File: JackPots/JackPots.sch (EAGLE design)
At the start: 20 parts, among them J101 F10, J102 F10, P1J0 JACK-3_5MM-MONO-SW-WQP_PJ302-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, P1JI JACK-3_5MM-MONO-SW-WQP_PJ302-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, P2J0 JACK-3_5MM-MONO-SW-WQP_PJ302-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, P2JI JACK-3_5MM-MONO-SW-WQP_PJ302-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, P3JI JACK-3_5MM-MONO-SW-WQP_PJ302-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, P3JO JACK-3_5MM-MONO-SW-WQP_PJ302-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, P4JI JACK-3_5MM-MONO-SW-WQP_PJ302-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, P4JO JACK-3_5MM-MONO-SW-WQP_PJ302-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

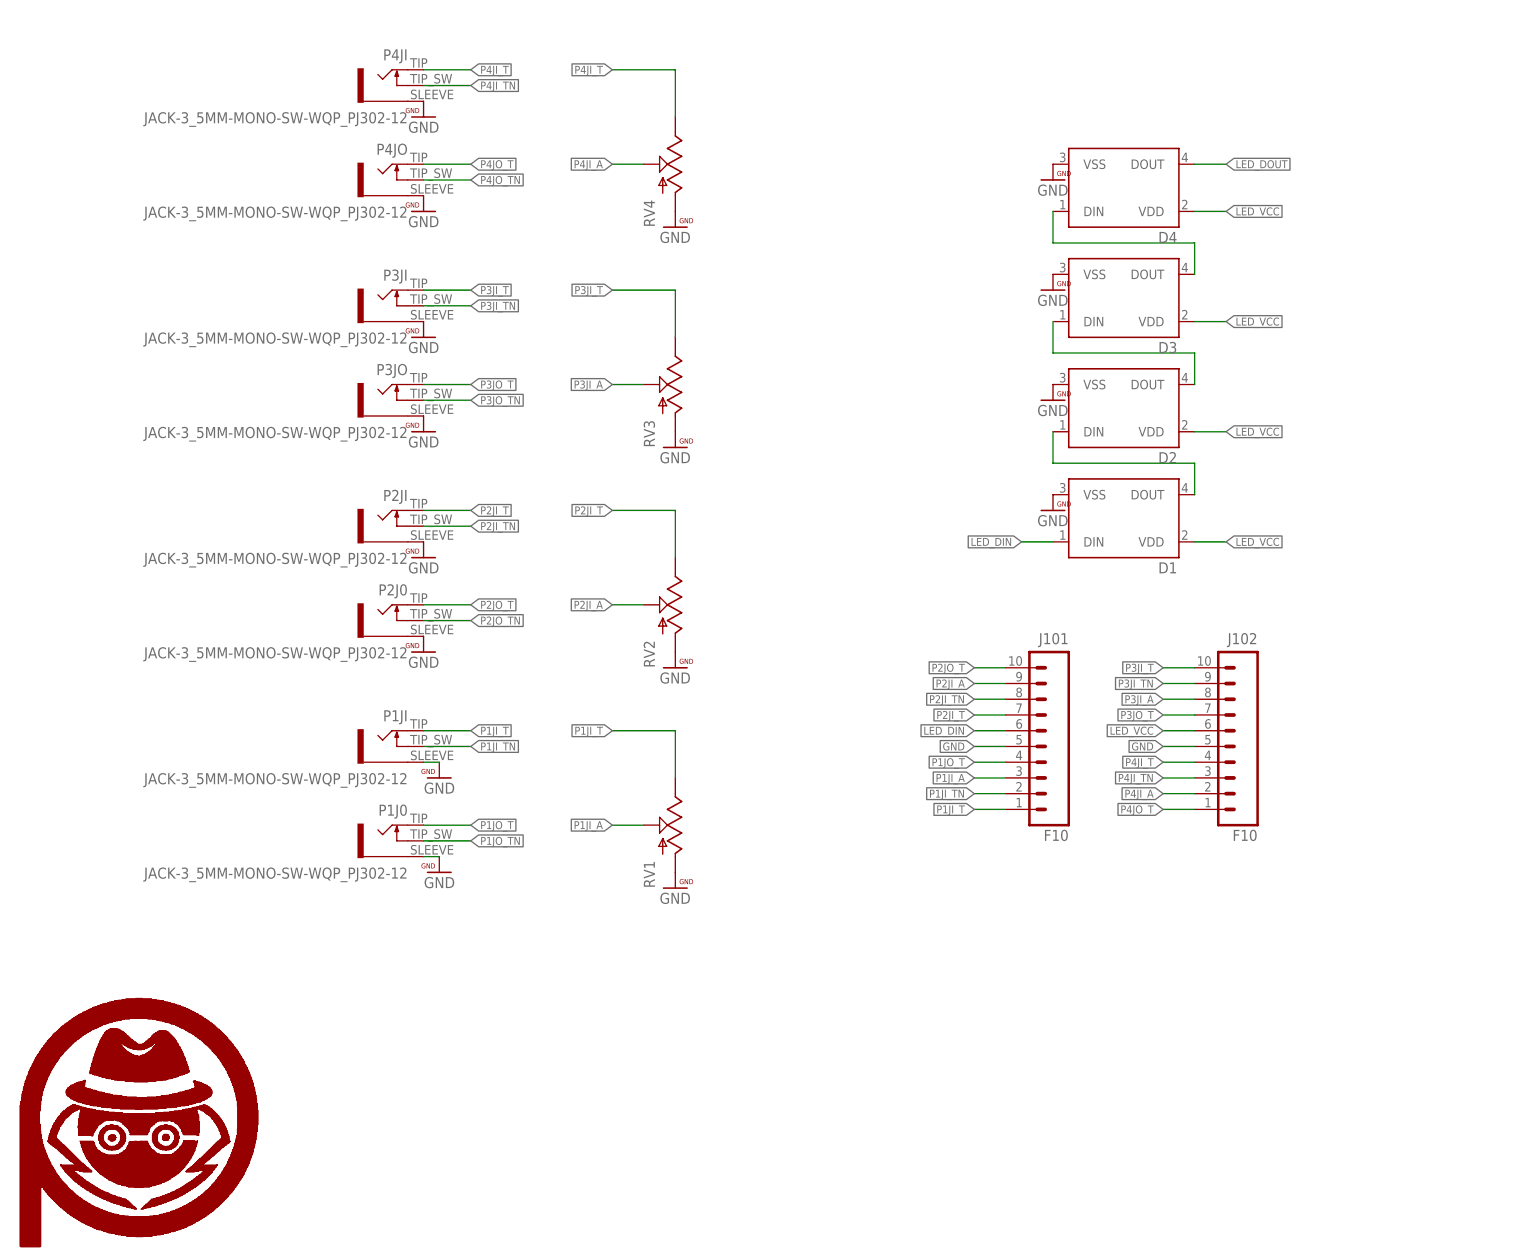
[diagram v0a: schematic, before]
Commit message: 4/10 update
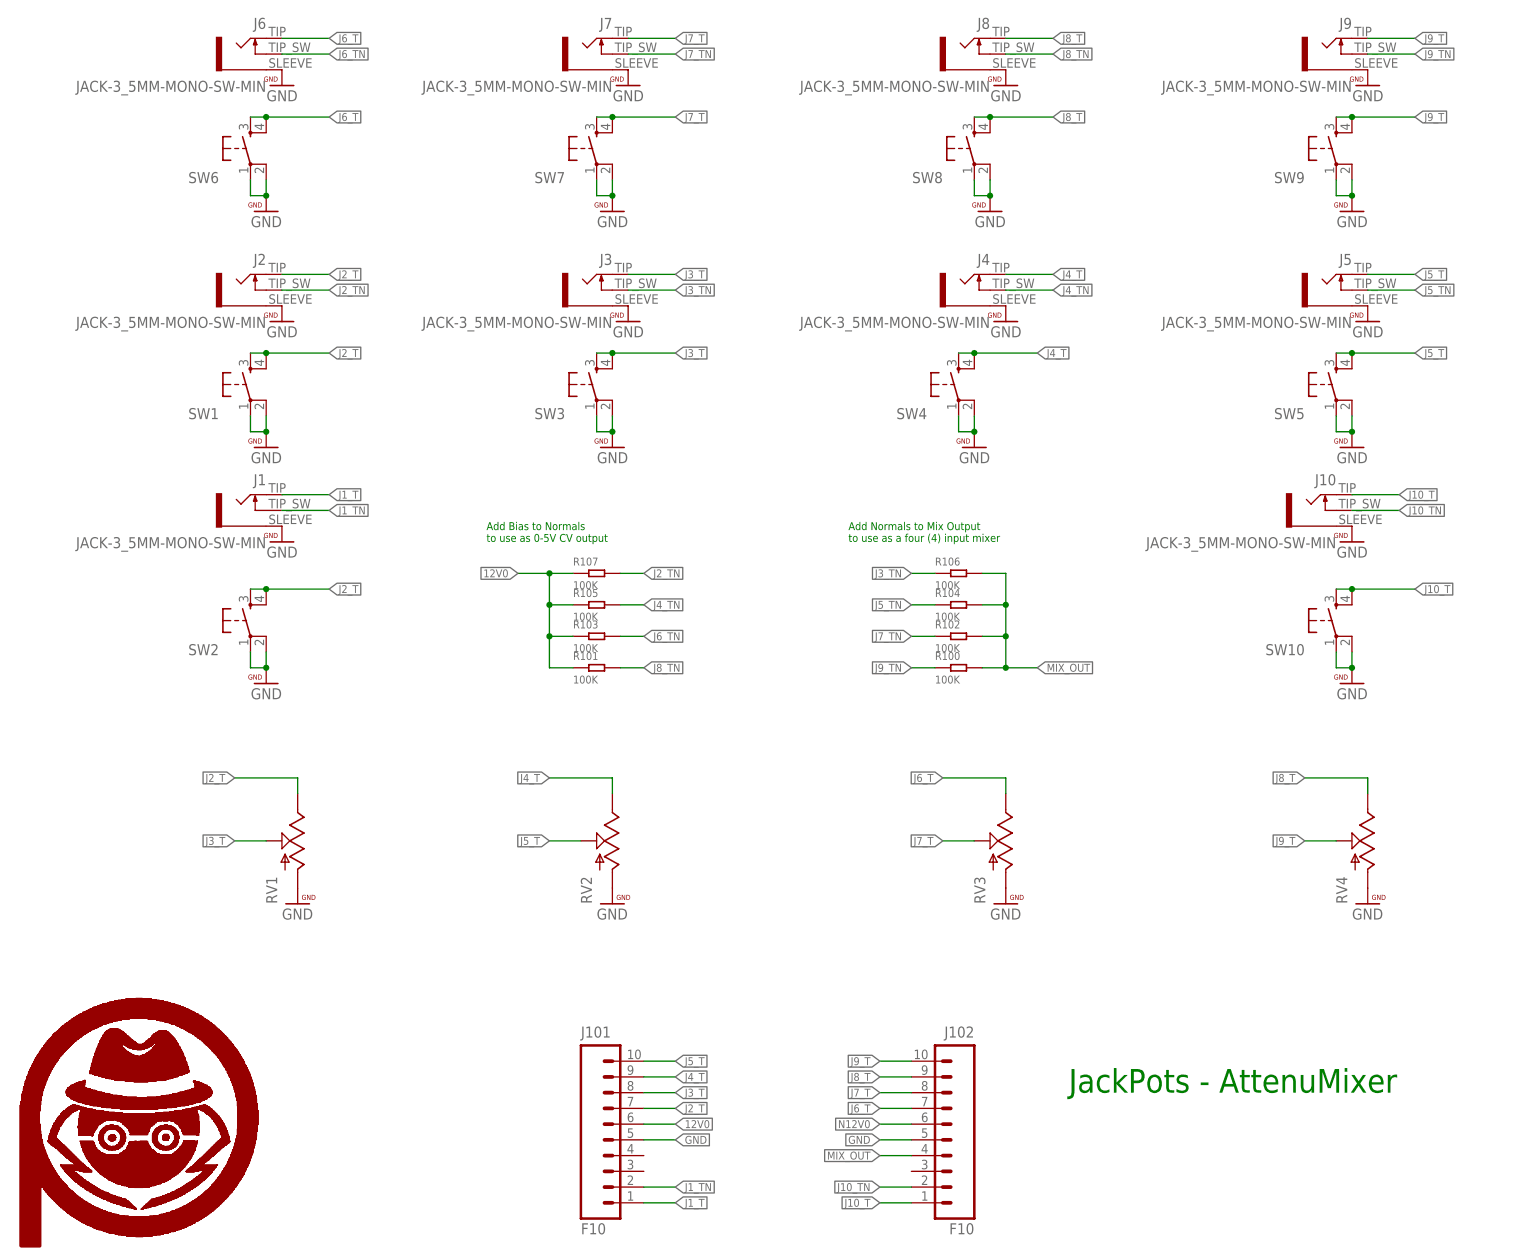
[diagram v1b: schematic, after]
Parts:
- removed D1, D2, D3, D4: (no value), halcyonmod_Optoelectronics:WS2812B-PTH
- removed P1J0, P1JI, P2J0, P2JI, P3JI, P3JO, P4JI, P4JO: JACK-3_5MM-MONO-SW-WQP_PJ302-12, oXo_Connectors:JACK-3_5MM-MONO-SW-WQP_PJ302-12
- removed U$16, U$18: PA_LOGO_SYMMED, PatternAgents-Logos:PA_LOGO_SYMMED
- added $$U$1: PA_LOGO_SYMSMALL, PatternAgents-Logos:PA_LOGO_SYMSMALL
- added $$U$100, $$U$101: PA_LOGO_SYMMED, PatternAgents-Logos:PA_LOGO_SYMMED
- added J1, J10, J2, J3, J4, J5, J6, J7, J8, J9: JACK-3_5MM-MONO-SW-MIN, halcyonmod_Connectors:JACK-3_5MM-MONO-SW-MIN
- added R100, R101, R102, R103, R104, R105, R106, R107: 100K, Seeed-Resistor-2016:SMD-RES-100K-1%-1/10W(0603)
- added SW1, SW10, SW2, SW3, SW4, SW5, SW6, SW7, SW8, SW9: (no value), SparkFun:TAC_SWITCHPTH
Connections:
- removed net LED_DIN: D1.DIN, J101.6
- removed net LED_DOUT: D4.DOUT
- removed net LED_VCC: D1.VDD, D2.VDD, D3.VDD, D4.VDD, J102.6
- removed net N$1: D1.DOUT, D2.DIN
- removed net N$2: D2.DOUT, D3.DIN
- removed net N$3: D3.DOUT, D4.DIN
- removed net P1JI_A: J101.3, RV1.2
- removed net P1JI_T: J101.1, P1JI.TIP, RV1.3
- removed net P1JI_TN: J101.2, P1JI.TIP_SW
- removed net P1JO_T: J101.4, P1J0.TIP
- removed net P1JO_TN: P1J0.TIP_SW
- removed net P2JI_A: J101.9, RV2.2
- removed net P2JI_T: J101.7, P2JI.TIP, RV2.3
- removed net P2JI_TN: J101.8, P2JI.TIP_SW
- removed net P2JO_T: J101.10, P2J0.TIP
- removed net P2JO_TN: P2J0.TIP_SW
- removed net P3JI_A: J102.8, RV3.2
- removed net P3JI_T: J102.10, P3JI.TIP, RV3.3
- removed net P3JI_TN: J102.9, P3JI.TIP_SW
- removed net P3JO_T: J102.7, P3JO.TIP
- removed net P3JO_TN: P3JO.TIP_SW
- removed net P4JI_A: J102.2, RV4.2
- removed net P4JI_T: J102.4, P4JI.TIP, RV4.3
- removed net P4JI_TN: J102.3, P4JI.TIP_SW
- removed net P4JO_T: J102.1, P4JO.TIP
- removed net P4JO_TN: P4JO.TIP_SW
- new net 12V0: J101.6, R101.1, R103.1, R105.1, R107.1
- new net J10_T: J10.TIP, J102.1, SW10.3, SW10.4
- new net J10_TN: J10.TIP_SW, J102.2
- new net J1_T: J1.TIP, J101.1
- new net J1_TN: J1.TIP_SW, J101.2
- new net J2_T: J101.7, J2.TIP, RV1.3, SW1.3, SW1.4, SW2.3, SW2.4
- new net J2_TN: J2.TIP_SW, R107.2
- new net J3_T: J101.8, J3.TIP, RV1.2, SW3.3, SW3.4
- new net J3_TN: J3.TIP_SW, R106.1
- new net J4_T: J101.9, J4.TIP, RV2.3, SW4.3, SW4.4
- new net J4_TN: J4.TIP_SW, R105.2
- new net J5_T: J101.10, J5.TIP, RV2.2, SW5.3, SW5.4
- new net J5_TN: J5.TIP_SW, R104.1
- new net J6_T: J102.7, J6.TIP, RV3.3, SW6.3, SW6.4
- new net J6_TN: J6.TIP_SW, R103.2
- new net J7_T: J102.8, J7.TIP, RV3.2, SW7.3, SW7.4
- new net J7_TN: J7.TIP_SW, R102.1
- new net J8_T: J102.9, J8.TIP, RV4.3, SW8.3, SW8.4
- new net J8_TN: J8.TIP_SW, R101.2
- new net J9_T: J102.10, J9.TIP, RV4.2, SW9.3, SW9.4
- new net J9_TN: J9.TIP_SW, R100.1
- new net MIX_OUT: J102.4, R100.2, R102.2, R104.2, R106.2
- new net N12V0: J102.6
- net GND: now also J1.SLEEVE, J10.SLEEVE, J2.SLEEVE, J3.SLEEVE, J4.SLEEVE, J5.SLEEVE, J6.SLEEVE, J7.SLEEVE, J8.SLEEVE, J9.SLEEVE, SW1.1, SW1.2, SW10.1, SW10.2, SW2.1, SW2.2, SW3.1, SW3.2, SW4.1, SW4.2, SW5.1, SW5.2, SW6.1, SW6.2, SW7.1, SW7.2, SW8.1, SW8.2, SW9.1, SW9.2; no longer D1.VSS, D2.VSS, D3.VSS, D4.VSS, P1J0.SLEEVE, P1JI.SLEEVE, P2J0.SLEEVE, P2JI.SLEEVE, P3JI.SLEEVE, P3JO.SLEEVE, P4JI.SLEEVE, P4JO.SLEEVE
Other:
- note added: "Add Bias to Normals to use as 0-5V CV output"
- note added: "Add Normals to Mix Output to use as a four (4) input mixer"
- note added: "JackPots - AttenuMixer"
- moved on the sheet: J101, J102, RV1, RV2, RV3, RV4
